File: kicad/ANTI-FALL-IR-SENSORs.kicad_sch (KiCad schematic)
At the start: 10 parts, among them J4 ANTI-FALL-LEFT-DOWN, J5 ANTI-FALL-RIGHT-DOWN

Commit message: Changed MCU to STM32G473VCT6
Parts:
- R67, R68, R69, R70, R71, R72, R73, R74: footprint oomwoo_altium:RES-0402 -> Resistor_SMD:R_0603_1608Metric
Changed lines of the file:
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@@
 			)
 		)
-		(property "Footprint" "oomwoo_altium:RES-0402"
+		(property "Footprint" "Resistor_SMD:R_0603_1608Metric"
 			(at 177.165 227.33 0)
 			(hide yes)
@@
 			)
 		)
-		(property "Footprint" "oomwoo_altium:RES-0402"
+		(property "Footprint" "Resistor_SMD:R_0603_1608Metric"
 			(at 332.105 247.65 0)
 			(hide yes)
@@
 			)
 		)
-		(property "Footprint" "oomwoo_altium:RES-0402"
+		(property "Footprint" "Resistor_SMD:R_0603_1608Metric"
 			(at 319.405 153.67 0)
 			(hide yes)
@@
 			)
 		)
-		(property "Footprint" "oomwoo_altium:RES-0402"
+		(property "Footprint" "Resistor_SMD:R_0603_1608Metric"
 			(at 189.865 247.65 0)
 			(hide yes)
@@
 			)
 		)
-		(property "Footprint" "oomwoo_altium:RES-0402"
+		(property "Footprint" "Resistor_SMD:R_0603_1608Metric"
 			(at 319.405 227.33 0)
 			(hide yes)
@@
 			)
 		)
-		(property "Footprint" "oomwoo_altium:RES-0402"
+		(property "Footprint" "Resistor_SMD:R_0603_1608Metric"
 			(at 332.105 173.99 0)
 			(hide yes)
@@
 			)
 		)
-		(property "Footprint" "oomwoo_altium:RES-0402"
+		(property "Footprint" "Resistor_SMD:R_0603_1608Metric"
 			(at 177.165 153.67 0)
 			(hide yes)
@@
 			)
 		)
-		(property "Footprint" "oomwoo_altium:RES-0402"
+		(property "Footprint" "Resistor_SMD:R_0603_1608Metric"
 			(at 189.865 173.99 0)
 			(hide yes)

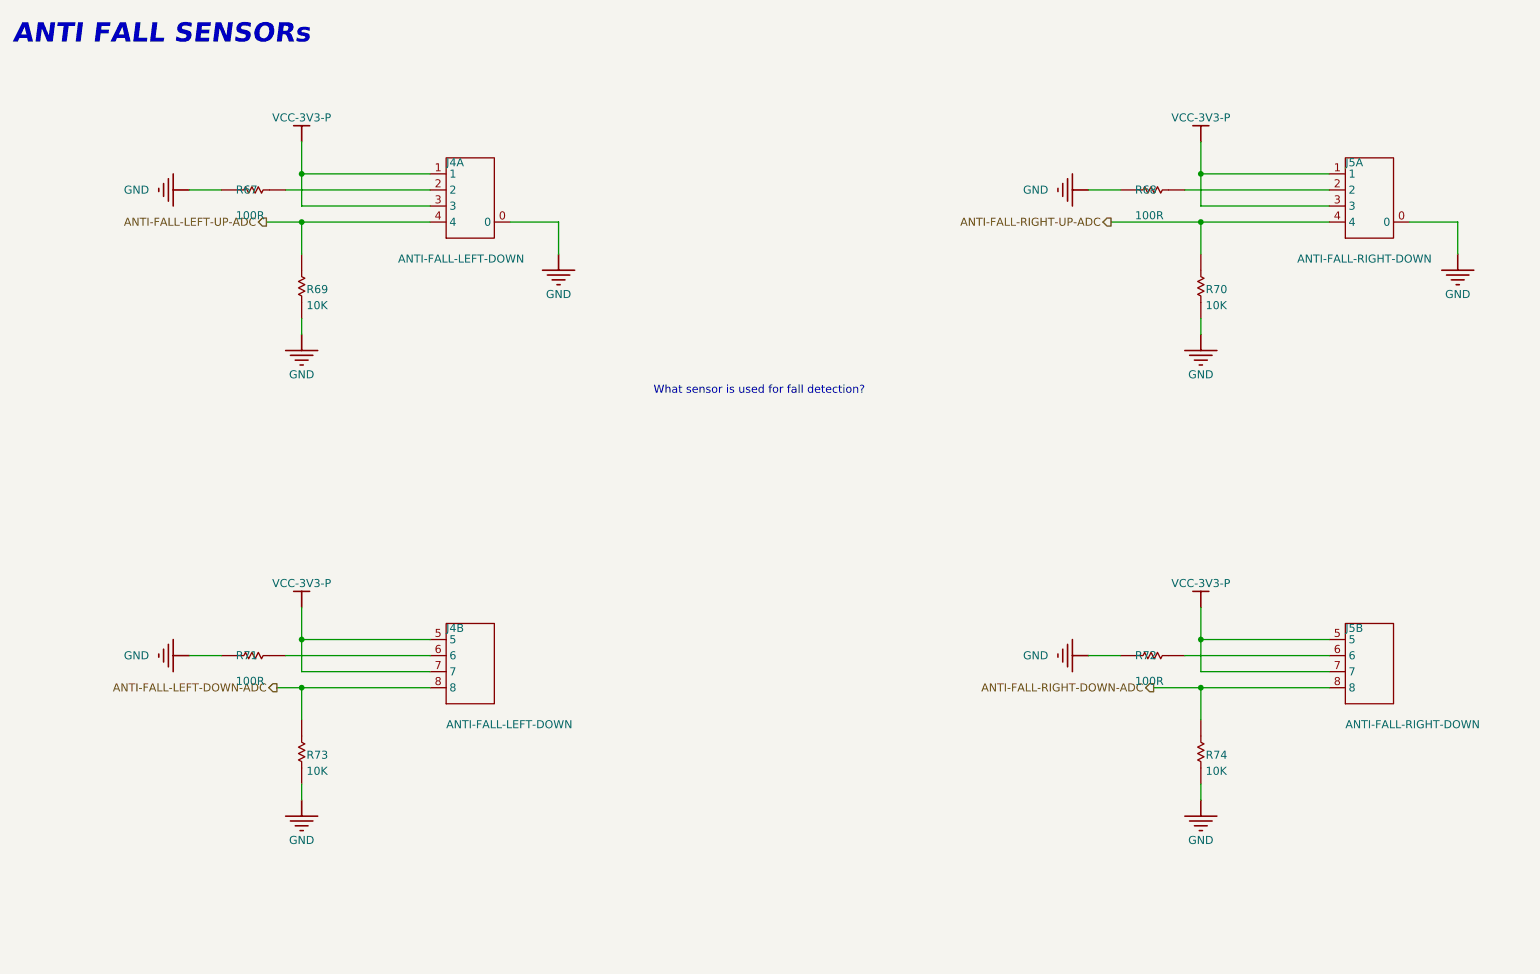
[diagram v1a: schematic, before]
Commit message: STM32G473VCT6
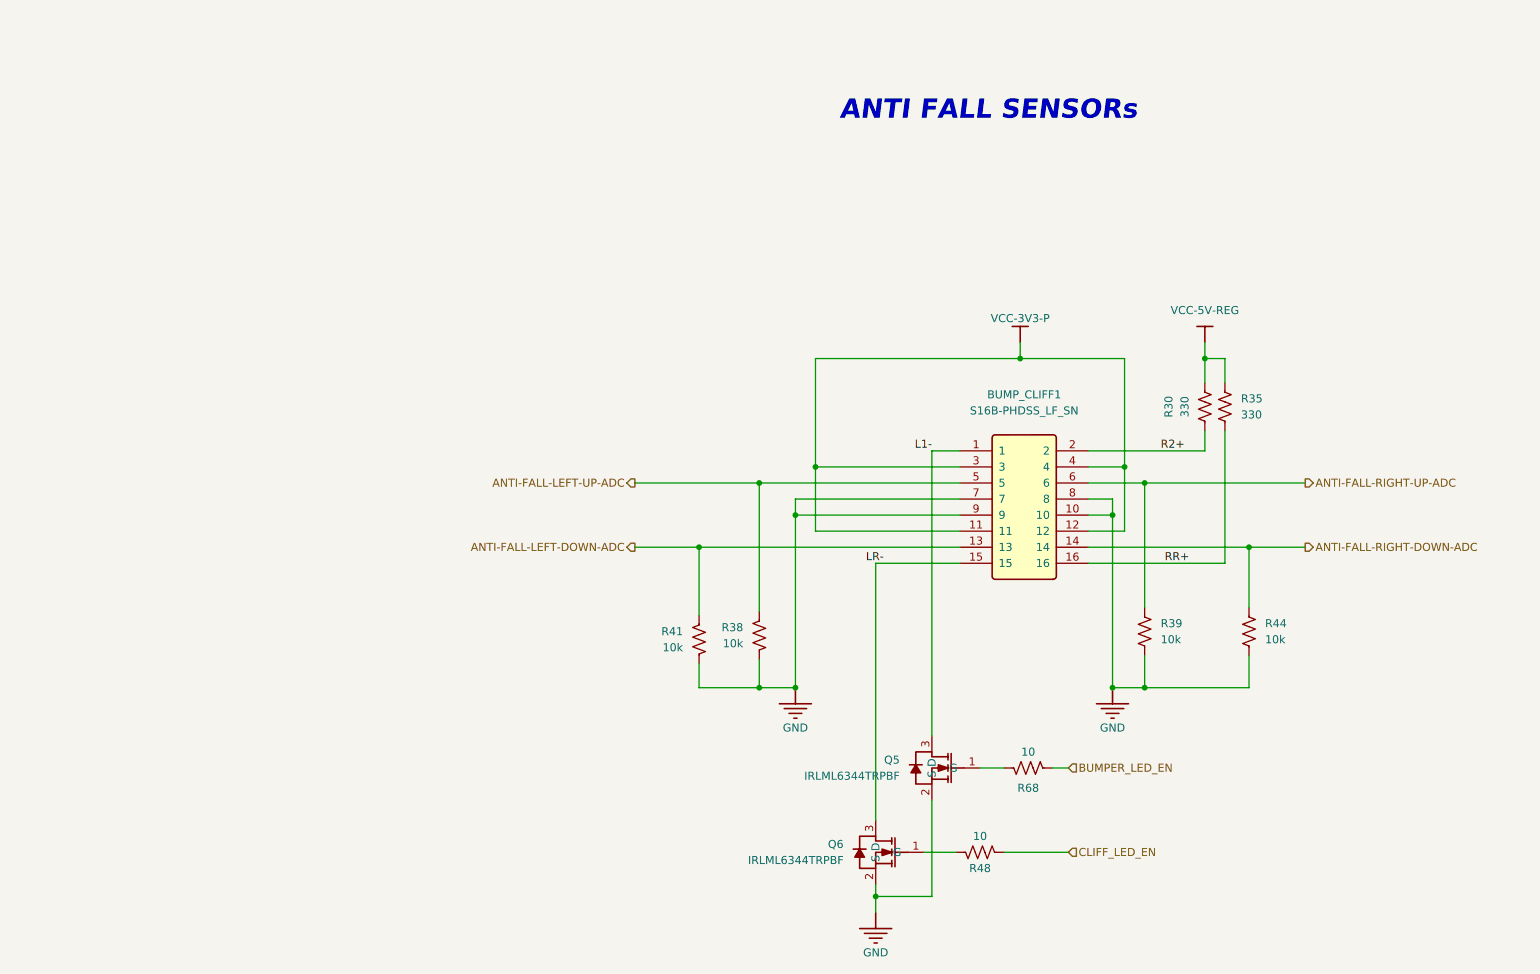
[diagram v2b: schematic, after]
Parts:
- removed J4: ANTI-FALL-LEFT-DOWN, oomwoo_altium:CONN-SMD_8P-P1.50_ZX-ZH1.5-8PWT, symbol DesignLibrary:ANTI-FALL_0_HDRx8-2_DesignLibrary.SchLib
- removed J5: ANTI-FALL-RIGHT-DOWN, oomwoo_altium:CONN-SMD_8P-P1.50_ZX-ZH1.5-8PWT, symbol DesignLibrary:ANTI-FALL_0_HDRx8-2_DesignLibrary.SchLib
- removed R67, R68, R71, R72: 100R, Resistor_SMD:R_0603_1608Metric, symbol DesignLibrary:ANTI-FALL_0_Resistor-1_DesignLibrary.SchLib
- removed R69, R70, R73, R74: 10K, Resistor_SMD:R_0603_1608Metric, symbol DesignLibrary:ANTI-FALL_1_Resistor-1_DesignLibrary.SchLib
- added BUMP_CLIFF1: S16B-PHDSS_LF_SN, JLCImport:S16B-PHDSS_LF_SN, symbol JLCImport:S16B-PHDSS_LF_SN
- added Q5, Q6: IRLML6344TRPBF, JLCImport:IRLML6344TRPBF, symbol JLCImport:IRLML6344TRPBF
- added R30, R35: 330, symbol Device:R_US
- added R38, R39, R41, R44: 10k, symbol Device:R_US
- added R48, R68: 10, Resistor_SMD:R_0603_1608Metric_Pad0.98x0.95mm_HandSolder, symbol Device:R_US
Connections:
- net ANTI-FALL-LEFT-DOWN-ADC: now also BUMP_CLIFF1.13, R41.1
- net ANTI-FALL-LEFT-UP-ADC: now also BUMP_CLIFF1.5, R38.1
- net ANTI-FALL-RIGHT-DOWN-ADC: now also BUMP_CLIFF1.14, R44.1
- net ANTI-FALL-RIGHT-UP-ADC: now also BUMP_CLIFF1.6, R39.1
- net GND: now also BUMP_CLIFF1.10, BUMP_CLIFF1.7, BUMP_CLIFF1.8, BUMP_CLIFF1.9, Q5.2 (S), Q6.2 (S), R38.2, R39.2, R41.2, R44.2
- net VCC-3V3-P: now also BUMP_CLIFF1.11, BUMP_CLIFF1.12, BUMP_CLIFF1.3, BUMP_CLIFF1.4
- new net: Q6.1 (G), R48.2
- new net: Q5.1 (G), R68.2
- new net BUMPER_LED_EN: R68.1
- new net CLIFF_LED_EN: R48.1
- new net L1-: BUMP_CLIFF1.1, Q5.3 (D)
- new net LR-: BUMP_CLIFF1.15, Q6.3 (D)
- new net R2+: BUMP_CLIFF1.2, R30.1
- new net RR+: BUMP_CLIFF1.16, R35.1
- new net VCC-5V-REG: R30.2, R35.2
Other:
- note removed: "What sensor is used for fall detection?"
